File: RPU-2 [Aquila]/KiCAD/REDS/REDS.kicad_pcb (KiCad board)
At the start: 4 copper layers, 40.5 x 37.5 mm, 14 parts, among them J3 REDS Power, J4 Our Stuff, M1 Servo, U3 LM555xN, U4 MAX4544

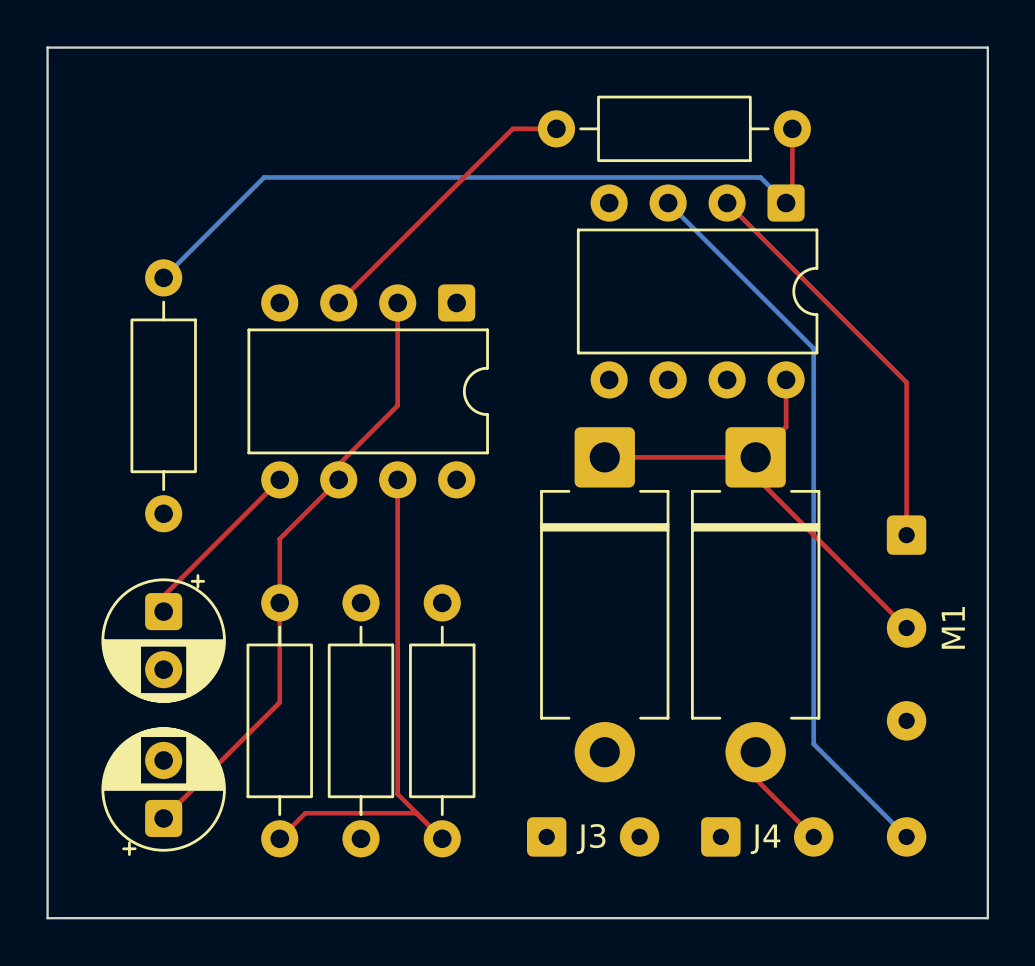
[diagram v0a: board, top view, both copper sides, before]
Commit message: pcb schematic
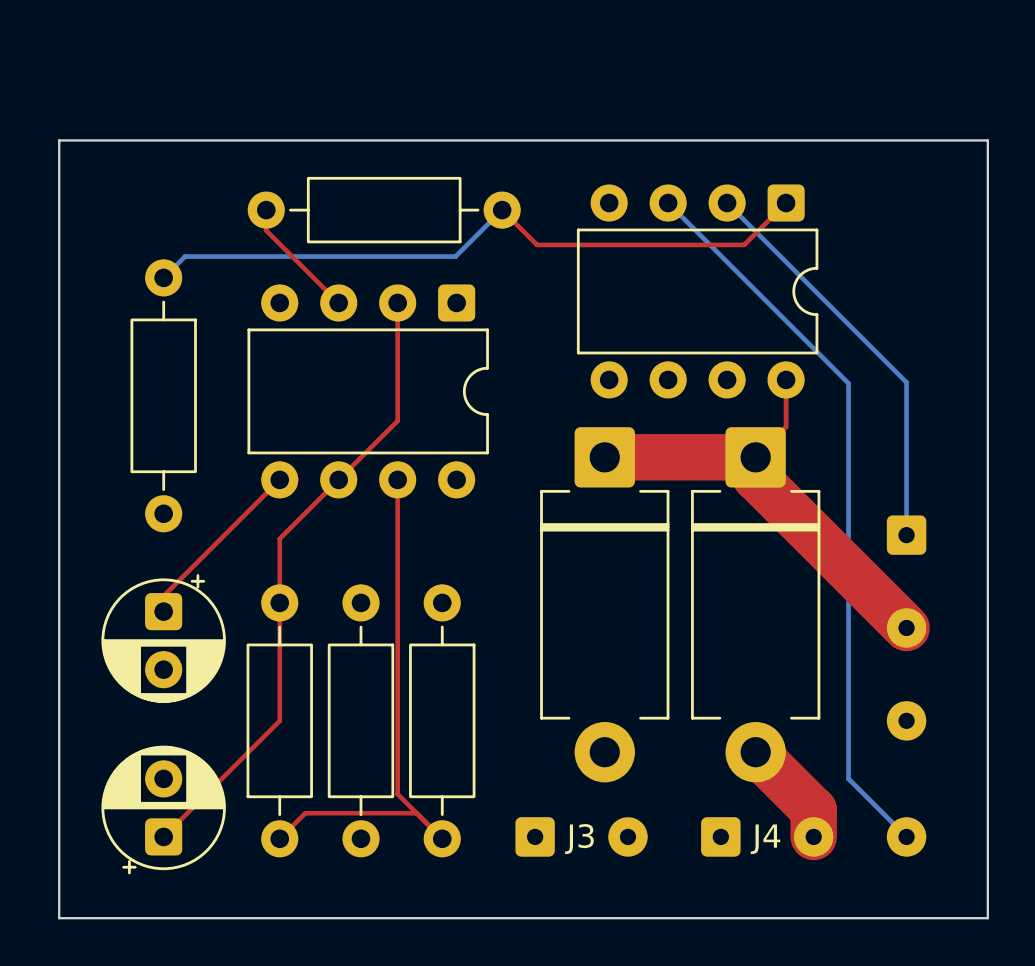
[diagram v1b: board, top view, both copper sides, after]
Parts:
- C1: value 100nF -> 1uF
- J3: value REDS Power -> Reds Power
- M1: value Servo -> Motor_Servo
- moved R5 13.0 mm to (116.1, 126.5)
- moved C1 0.79 mm to (101.5, 153.5)
- moved J3 0.50 mm to (117.5, 153.5)
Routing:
- net Net-(U3-Q): track 12.5 -> 5.29 mm
- net 555out: track 32.4 -> 29.4 mm
- net Net-(U3-THR): track 26.4 -> 27.2 mm
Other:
- board size 40.5 x 37.5 mm -> 40 x 33.5 mm
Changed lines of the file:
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@@
 			(at 4 -2.05 90)
 			(layer "F.SilkS")
+			(hide yes)
 			(effects
 				(font
@@
 			)
 		)
-		(property "Value" "Servo"
-			(at 4 2.05 90)
+		(property "Value" "Motor_Servo"
+			(at 4 -2.5 90)
 			(layer "F.Fab")
 			(effects
@@
 			(pinfunction "-_3")
 			(pintype "passive")
+			(thermal_bridge_width 1)
 		)
 		(embedded_fonts no)
@@
 		)
 		(property "Value" "1nF"
-			(at 1.25 3.75 90)
+			(at -2.294887 0 180)
 			(layer "F.Fab")
 			(effects
@@
 			(pinfunction "A_2")
 			(pintype "passive")
+			(thermal_bridge_width 1)
 		)
 		(embedded_fonts no)
@@
 	(footprint "Connector_Wire:SolderWire-0.15sqmm_1x02_P4mm_D0.5mm_OD1.5mm"
 		(layer "F.Cu")
-		(at 118 153.5)
+		(at 117.5 153.5)
 		(descr "Soldered wire connection, for 2 times 0.15 mm² wires, basic insulation, conductor diameter 0.5mm, outer diameter 1.5mm, size source Multi-Contact FLEXI-E 0.15 (https://www.staubli.com/content/dam/ecs/catalogs-brochures/TM/CAB-Main-11014119-en.pdf#page=9), bend radius 3 times outer diameter")
 		(tags "connector wire 0.15sqmm")
@@
 			)
 		)
-		(property "Value" "REDS Power"
-			(at 2 2 0)
+		(property "Value" "Reds Power"
+			(at 2 2.5 0)
 			(layer "F.Fab")
 			(effects
@@
 			(pinfunction "Pin_1_1")
 			(pintype "passive")
+			(thermal_bridge_width 1)
 		)
 		(pad "2" thru_hole circle
@@
 			(pinfunction "Pin_2_2")
 			(pintype "passive")
+			(thermal_bridge_width 1)
 		)
 		(embedded_fonts no)
@@
 	(footprint "Resistor_THT:R_Axial_DIN0207_L6.3mm_D2.5mm_P10.16mm_Horizontal"
 		(layer "F.Cu")
-		(at 128.58 123 180)
+		(at 116.08 126.5 180)
 		(descr "Resistor, Axial_DIN0207 series, Axial, Horizontal, pin pitch=10.16mm, 0.25W = 1/4W, length*diameter=6.3*2.5mm^2, http://cdn-reichelt.de/documents/datenblatt/B400/1_4W%23YAG.pdf")
 		(tags "Resistor Axial_DIN0207 series Axial Horizontal pin pitch 10.16mm 0.25W = 1/4W length 6.3mm diameter 2.5mm")
@@
 		)
 		(property "Value" "Our Stuff"
-			(at 4 2.05 0)
+			(at 4.5 2.5 0)
 			(layer "F.Fab")
 			(effects
@@
 			(pinfunction "Pin_1_1")
 			(pintype "passive")
+			(thermal_bridge_width 1)
 		)
 		(pad "2" thru_hole circle
@@
 	(footprint "Capacitor_THT:CP_Radial_D5.0mm_P2.50mm"
 		(layer "F.Cu")
-		(at 101.5 152.705112 90)
+		(at 101.5 153.5 90)
 		(descr "CP, Radial series, Radial, pin pitch=2.50mm, diameter=5mm, height=7mm, Electrolytic Capacitor")
 		(tags "CP Radial series Radial pin pitch 2.50mm diameter 5mm height 7mm Electrolytic Capacitor")
@@
 			)
 		)
-		(property "Value" "100nF"
-			(at 1.205112 -3.5 270)
+		(property "Value" "1uF"
+			(at 5 0 0)
 			(layer "F.Fab")
 			(effects
@@
 	)
 	(gr_rect
-		(start 96.5 119.5)
+		(start 97 123.5)
 		(end 137 157)
 		(stroke
@@
 	(segment
 		(start 133.5 133.925)
-		(end 125.77 126.195)
+		(end 133.5 140.5)
 		(width 0.2)
-		(layer "F.Cu")
+		(layer "B.Cu")
 		(net "Net-(M1-PWM)")
 	)
 	(segment
-		(start 133.5 140.5)
+		(start 125.77 126.195)
 		(end 133.5 133.925)
 		(width 0.2)
-		(layer "F.Cu")
+		(layer "B.Cu")
 		(net "Net-(M1-PWM)")
 	)
 	(segment
-		(start 127 138)
-		(end 133.5 144.5)
-		(width 0.2)
-		(layer "F.Cu")
-		(net "Net-(D1-K)")
-	)
-	(segment
-		(start 128.31 133.815)
-		(end 128.31 135.84)
-		(width 0.2)
-		(layer "F.Cu")
-		(net "Net-(D1-K)")
-	)
-	(segment
-		(start 128.31 135.84)
-		(end 127 137.15)
-		(width 0.2)
-		(layer "F.Cu")
-		(net "Net-(D1-K)")
-	)
-	(segment
-		(start 127 137.15)
-		(end 127 138)
-		(width 0.2)
-		(layer "F.Cu")
-		(net "Net-(D1-K)")
-	)
-	(segment
-		(start 120.5 137.15)
-		(end 127 137.15)
-		(width 0.2)
-		(layer "F.Cu")
-		(net "Net-(D1-K)")
-	)
-	(segment
 		(start 107.6 152.48)
 		(end 112.4 152.48)
@@
 	)
 	(segment
-		(start 113.5 153.58)
-		(end 111.58 151.66)
+		(start 111.58 151.66)
+		(end 113.5 153.58)
 		(width 0.2)
 		(layer "F.Cu")
@@
 	)
 	(segment
-		(start 111.58 151.66)
-		(end 111.58 138.12)
+		(start 111.58 138.12)
+		(end 111.58 151.66)
 		(width 0.2)
 		(layer "F.Cu")
@@
 	)
 	(segment
-		(start 112.4 152.48)
-		(end 113.5 153.58)
+		(start 106.5 153.58)
+		(end 107.6 152.48)
 		(width 0.2)
 		(layer "F.Cu")
@@
 	)
 	(segment
-		(start 106.5 153.58)
-		(end 107.6 152.48)
+		(start 112.4 152.48)
+		(end 113.5 153.58)
 		(width 0.2)
 		(layer "F.Cu")
@@
 	)
 	(segment
-		(start 101.5 143.12)
-		(end 101.5 143.794887)
+		(start 101.5 143.794887)
+		(end 101.5 143.12)
 		(width 0.2)
 		(layer "F.Cu")
@@
 	)
 	(segment
-		(start 106.5 138.12)
-		(end 101.5 143.12)
+		(start 101.5 143.12)
+		(end 106.5 138.12)
 		(width 0.2)
 		(layer "F.Cu")
@@
 	)
 	(segment
-		(start 101.5 152.705112)
-		(end 106.5 147.705112)
+		(start 111.58 135.58)
+		(end 109.04 138.12)
 		(width 0.2)
 		(layer "F.Cu")
@@
 	)
 	(segment
-		(start 109.04 138.12)
-		(end 109.04 137.46)
+		(start 106.5 140.66)
+		(end 109.04 138.12)
 		(width 0.2)
 		(layer "F.Cu")
@@
 	)
 	(segment
-		(start 106.5 147.705112)
-		(end 106.5 143.42)
+		(start 106.5 148.5)
+		(end 101.5 153.5)
 		(width 0.2)
 		(layer "F.Cu")
@@
 	)
 	(segment
-		(start 109.04 137.46)
-		(end 111.58 134.92)
+		(start 111.58 130.5)
+		(end 111.58 135.58)
 		(width 0.2)
 		(layer "F.Cu")
@@
 	)
 	(segment
-		(start 111.58 134.92)
-		(end 111.58 130.5)
+		(start 106.5 143.42)
+		(end 106.5 148.5)
 		(width 0.2)
 		(layer "F.Cu")
@@
 	)
 	(segment
-		(start 106.5 140.66)
-		(end 109.04 138.12)
+		(start 128.31 126.195)
+		(end 126.505 128)
 		(width 0.2)
 		(layer "F.Cu")
-		(net "Net-(U3-THR)")
+		(net "555out")
 	)
 	(segment
-		(start 128.58 125.925)
-		(end 128.31 126.195)
+		(start 117.58 128)
+		(end 116.08 126.5)
 		(width 0.2)
 		(layer "F.Cu")
@@
 	)
 	(segment
-		(start 128.58 123)
-		(end 128.58 125.925)
+		(start 126.505 128)
+		(end 117.58 128)
 		(width 0.2)
 		(layer "F.Cu")
@@
 	)
 	(segment
-		(start 127.21 125.095)
-		(end 105.825 125.095)
+		(start 114.08 128.5)
+		(end 102.42 128.5)
 		(width 0.2)
 		(layer "B.Cu")
@@
 	)
 	(segment
-		(start 128.31 126.195)
-		(end 127.21 125.095)
+		(start 116.08 126.5)
+		(end 114.08 128.5)
 		(width 0.2)
 		(layer "B.Cu")
@@
 	)
 	(segment
-		(start 105.825 125.095)
+		(start 102.42 128.5)
 		(end 101.5 129.42)
 		(width 0.2)
@@
 	)
 	(segment
-		(start 129.5 149.5)
-		(end 133.5 153.5)
+		(start 131 133.965)
+		(end 123.23 126.195)
 		(width 0.2)
 		(layer "B.Cu")
@@
 	)
 	(segment
-		(start 129.5 132.465)
-		(end 129.5 149.5)
+		(start 133.5 153.5)
+		(end 131 151)
 		(width 0.2)
 		(layer "B.Cu")
@@
 	)
 	(segment
-		(start 123.23 126.195)
-		(end 129.5 132.465)
+		(start 131 151)
+		(end 131 133.965)
 		(width 0.2)
 		(layer "B.Cu")
@@
 	)
 	(segment
-		(start 116.54 123)
-		(end 118.42 123)
+		(start 109.04 130.5)
+		(end 105.92 127.38)
 		(width 0.2)
 		(layer "F.Cu")
@@
 	)
 	(segment
-		(start 109.04 130.5)
-		(end 116.54 123)
+		(start 105.92 127.38)
+		(end 105.92 126.5)
 		(width 0.2)
 		(layer "F.Cu")
@@
 	)
 	(segment
-		(start 127 151)
+		(start 129.5 152.35)
 		(end 127 149.85)
-		(width 0.2)
+		(width 2)
 		(layer "F.Cu")
 		(net "OurPower")
@@
 	(segment
 		(start 129.5 153.5)
-		(end 127 151)
-		(width 0.2)
+		(end 129.5 152.35)
+		(width 2)
 		(layer "F.Cu")
 		(net "OurPower")
 	)
+	(segment
+		(start 127 138)
+		(end 133.5 144.5)
+		(width 2)
+		(layer "F.Cu")
+		(net "Net-(D1-K)")
+	)
+	(segment
+		(start 120.5 137.15)
+		(end 127 137.15)
+		(width 2)
+		(layer "F.Cu")
+		(net "Net-(D1-K)")
+	)
+	(segment
+		(start 128.31 133.815)
+		(end 128.31 135.84)
+		(width 0.2)
+		(layer "F.Cu")
+		(net "Net-(D1-K)")
+	)
+	(segment
+		(start 128.31 135.84)
+		(end 127 137.15)
+		(width 0.2)
+		(layer "F.Cu")
+		(net "Net-(D1-K)")
+	)
+	(segment
+		(start 127 137.15)
+		(end 127 138)
+		(width 2)
+		(layer "F.Cu")
+		(net "Net-(D1-K)")
+	)
 	(zone
 		(net "GND")
@@
 		(polygon
 			(pts
-				(xy 135 155) (xy 135 121.5) (xy 100 121.5) (xy 100 155)
+				(xy 135 155) (xy 135 125) (xy 99 125) (xy 99 155)
 			)
 		)
@@
 		(polygon
 			(pts
-				(xy 135 155) (xy 135 121.5) (xy 100 121.5) (xy 100 155)
+				(xy 135 155) (xy 135 125) (xy 99 125) (xy 99 155)
 			)
 		)
